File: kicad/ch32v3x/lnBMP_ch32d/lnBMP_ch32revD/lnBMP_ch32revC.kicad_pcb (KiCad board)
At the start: 2 copper layers, 52.6 x 33 mm, 29 parts, among them J1 BMP Debug1, J2 BMP Debug2, J3 Debug port, J4 USB_OTG, U1 CH32V303RCT6, U2 LM1117-3.3, Y1 Crystal, x2 PinSocket_1x03_P1.00mm_Vertic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

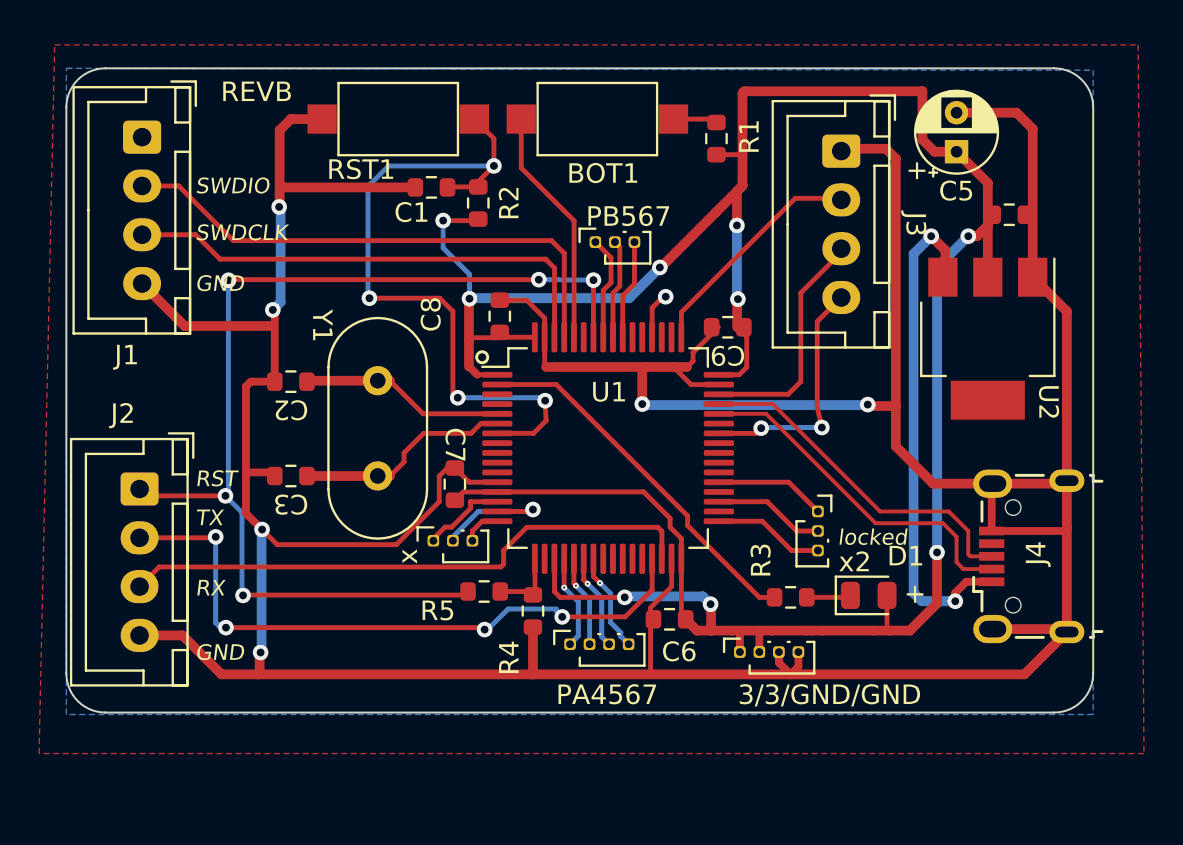
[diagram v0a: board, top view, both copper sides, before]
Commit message: new rev of ch32 pcb
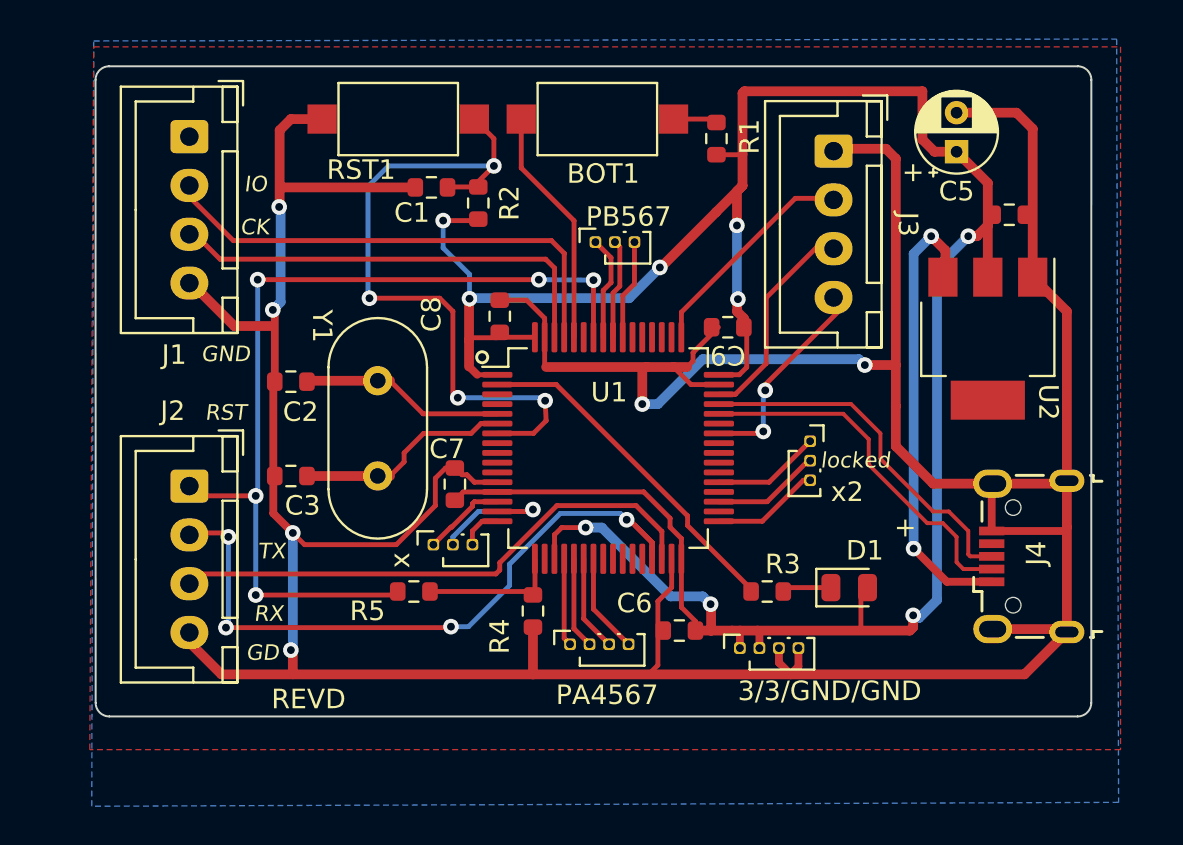
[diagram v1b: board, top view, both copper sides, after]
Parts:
- moved x2 3.62 mm to (140.9, 86.1)
- moved R5 3.60 mm to (120.6, 93.8)
- moved J2 2.55 mm to (109.1, 88.4)
- moved J1 2.42 mm to (109.1, 70.5)
- moved R3 1.24 mm to (138.7, 93.8)
- moved D1 1.08 mm to (142.9, 93.6)
- moved C6 0.76 mm to (134.2, 95.8)
- moved J3 0.39 mm to (142.1, 71.2)
- moved 3/3/GND/GND 0.20 mm to (137.3, 96.7)
- moved x 0.20 mm to (121.6, 91.4)
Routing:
- net INOUT_NRESET: track 54.6 -> 47.4 mm
- net GND: track 223.5 -> 216.5 mm
- net Net-(U1-PA3): track 3.12 -> 6.83 mm
- net unconnected-(U1-PC11-Pad52): track 2.75 -> 0.00 mm, vias 1 -> 0
- net Net-(J4-VBUS): track 25.8 -> 23.4 mm
- net OUT_UART_RX: track 29.9 -> 27.9 mm
- net UART_TX: track 12.6 -> 10.8 mm
- net OUT_SWDIO: track 27.4 -> 25.8 mm
- net OUT_SWDCLK: track 25.4 -> 23.8 mm
- net +3.3V: track 136.4 -> 137.9 mm
- net OUT_UART_TX: track 33.8 -> 35.3 mm
- net Net-(U1-PC13): track 19.0 -> 17.7 mm
- net SWDIO: track 12.3 -> 11.4 mm
- net D-: track 18.0 -> 18.8 mm
- net D+: track 17.9 -> 18.7 mm
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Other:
- board size 52.6 x 33 mm -> 51 x 33.3 mm
- board text added: "CK"
- board text added: "GD"
- board text added: "IO"
- board text added: "REVD"
- board text removed: "REVB"
- board text removed: "SWDCLK"
- board text removed: "SWDIO"
